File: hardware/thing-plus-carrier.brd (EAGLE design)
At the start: 160 x 100 mm, 8 parts, among them J1 THING_PLUS, U1 OKI-78SR-5/1.5-W36H-C, U2 MCP2004A-E/SNSOIC8_4P9X3P9MC_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, U3 MICROSD-BREAKOUT

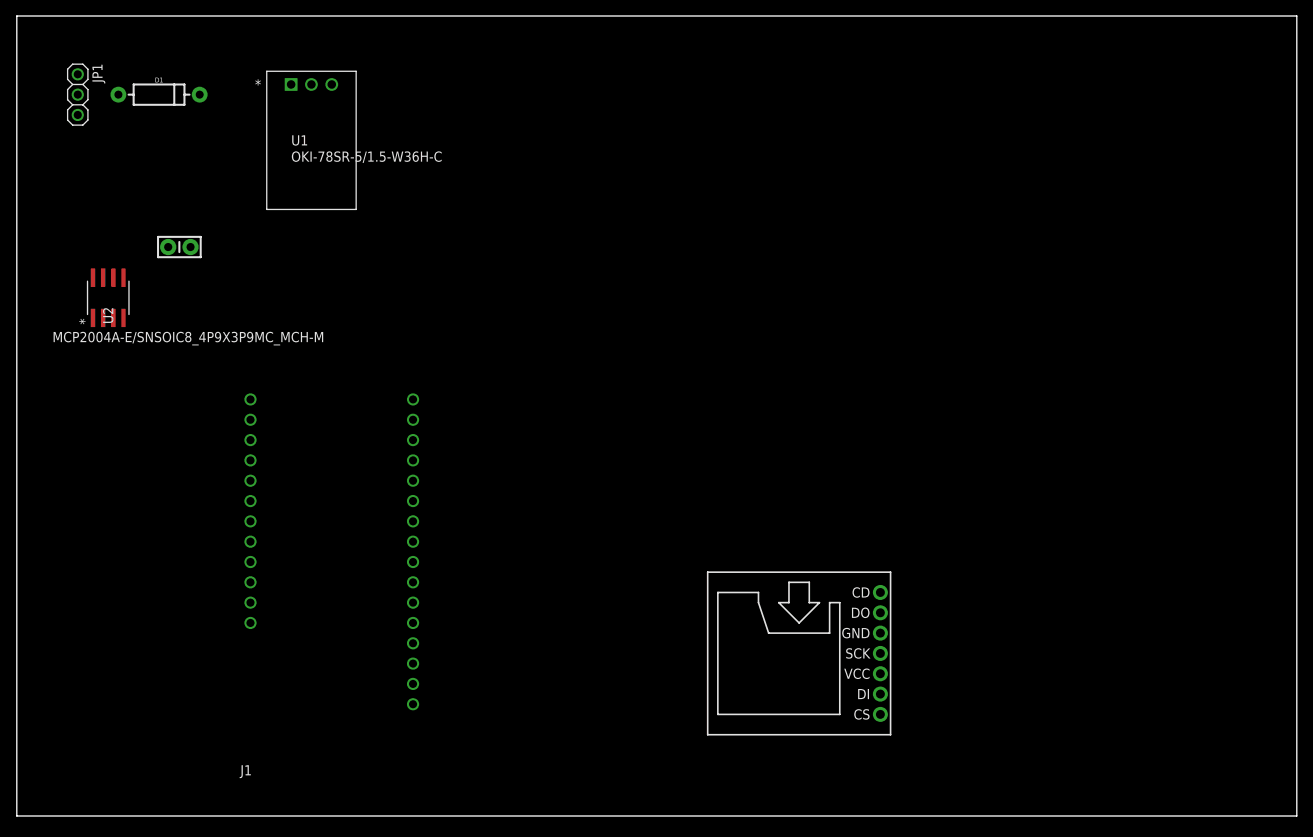
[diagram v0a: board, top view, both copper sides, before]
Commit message: Finished rev.1 board []~(￣▽￣)~* ; Updated docs
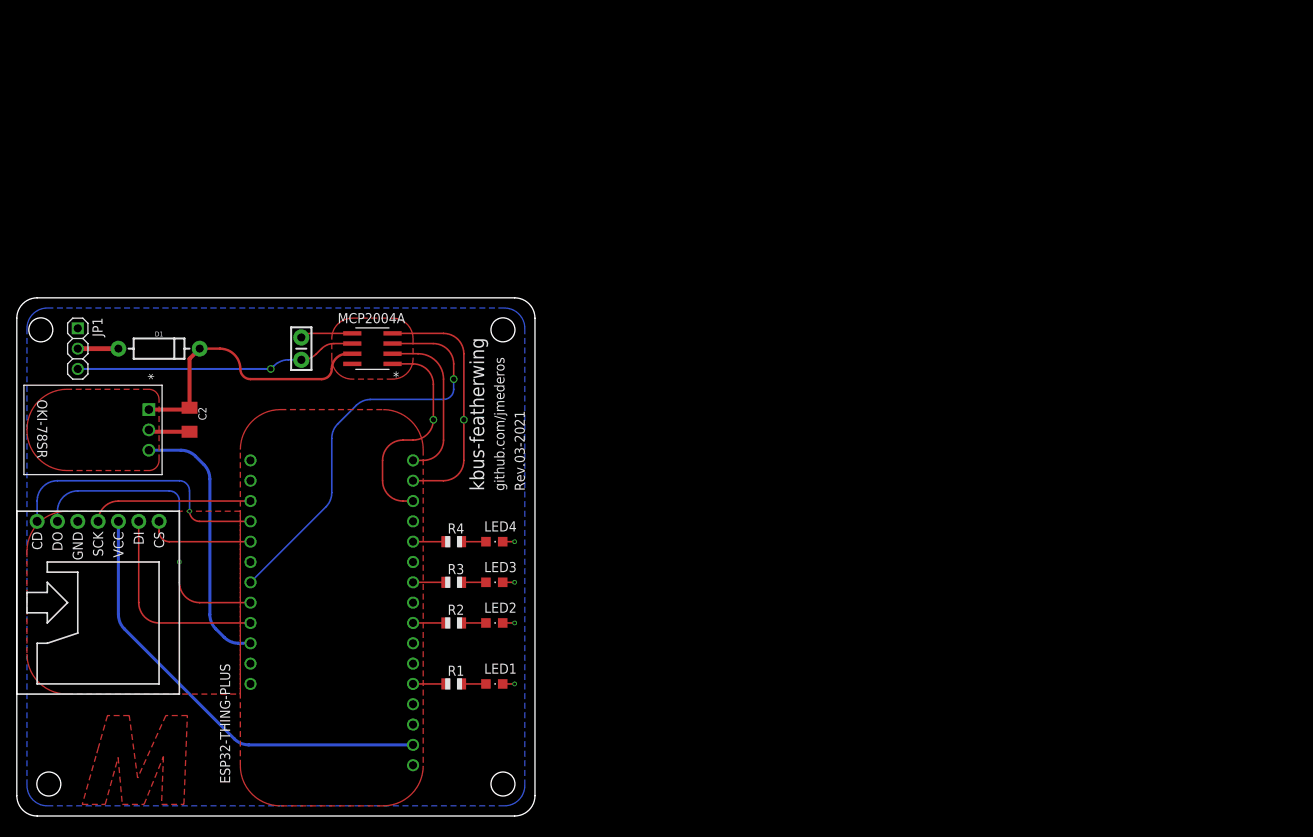
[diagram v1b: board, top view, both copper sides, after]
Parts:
- removed J1: THING_PLUS, SparkFun-Boards:THING_PLUS
- removed U1: OKI-78SR-5/1.5-W36H-C, kbus-feather-carrier-bom:OKI-78SR-5/1.5-W36H-C_MUR
- removed U2: MCP2004A-E/SNSOIC8_4P9X3P9MC_MCH-M, kbus-feather-carrier-bom:SOIC8_4P9X3P9MC_MCH-M
- added C2: 22uF, adafruit:C1206K
- added ESP32-THING-PLUS: THING_PLUS, SparkFun-Boards:THING_PLUS
- added LED1, LED2, LED3, LED4: (no value), adafruit:CHIPLED_0805
- added MCP2004A: MCP2004A-E/SNSOIC8_4P9X3P9MC_MCH-M, kbus-feather-carrier-bom:SOIC8_4P9X3P9MC_MCH-M
- added OKI-78SR: OKI-78SR-5/1.5-W36H-C, kbus-feather-carrier-bom:OKI-78SR-5/1.5-W36H-C_MUR
- added R1, R2, R3, R4: 1k, adafruit:R0805
- JP1: device adafruit:1X03 -> kbus-feather-carrier-bom:1X03
- U3: device SparkFun-Boards:MICROSD-BREAKOUT -> kbus-feather-carrier-bom:MICROSD-BREAKOUT
- moved U3 84.0 mm to (11.4, 24.1), turned to 90 degrees
- moved D1 31.8 mm to (17.8, 58.4)
- moved JP1 31.8 mm to (7.62, 58.4)
- moved C1 19.8 mm to (35.6, 58.4), turned to 90 degrees
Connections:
- new net N$1: ESP32-THING-PLUS.19, R3.1
- new net N$2: ESP32-THING-PLUS.24, R1.1
- new net N$3: ESP32-THING-PLUS.21, R2.1
- new net N$4: ESP32-THING-PLUS.17, R4.1
- new net N$5: LED4.A, R4.2
- new net N$6: LED3.A, R3.2
- new net N$7: LED2.A, R2.2
- new net N$8: LED1.A, R1.2
- net 12V: now also C2.1, MCP2004A.7, OKI-78SR.1; no longer U1.1, U2.7
- net 3V3: now also ESP32-THING-PLUS.27; no longer J1.27
- net 5V: now also ESP32-THING-PLUS.10, OKI-78SR.3; no longer J1.10, U1.3
- net CD: now also ESP32-THING-PLUS.4
- net CIPO: now also ESP32-THING-PLUS.8
- net COPI: now also ESP32-THING-PLUS.9
- net FAULT: now also ESP32-THING-PLUS.7, MCP2004A.3; no longer J1.7, U2.3
- net GND: now also C2.2, ESP32-THING-PLUS.25, ESP32-THING-PLUS.26, LED1.C, LED2.C, LED3.C, LED4.C, MCP2004A.5, OKI-78SR.2; no longer J1.25, J1.26, U1.2, U2.5
- net K-BUS: now also MCP2004A.6; no longer U2.6
- net RX: now also ESP32-THING-PLUS.15, MCP2004A.1; no longer J1.15, U2.1
- net SCK: now also ESP32-THING-PLUS.3
- net SD-CS: now also ESP32-THING-PLUS.5
- net TRX-CS: now also ESP32-THING-PLUS.13, MCP2004A.2; no longer J1.3, U2.2
- net TX: now also ESP32-THING-PLUS.14, MCP2004A.4; no longer J1.14, U2.4
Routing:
- net 3V3: track 0.00 -> 55.5 mm
- net FAULT: track 0.00 -> 52.0 mm, vias 0 -> 1
- net CIPO: track 0.00 -> 38.2 mm, vias 0 -> 1
- net 12V: track 0.00 -> 35.4 mm
- net K-BUS: track 0.00 -> 35.2 mm, vias 0 -> 1
- net CD: track 0.00 -> 33.9 mm, vias 0 -> 1
- net 5V: track 0.00 -> 33.2 mm
- net TX: track 0.00 -> 30.7 mm, vias 0 -> 1
- net RX: track 0.00 -> 26.5 mm, vias 0 -> 1
- net COPI: track 0.00 -> 25.2 mm
- net TRX-CS: track 0.00 -> 20.2 mm
- net SCK: track 0.00 -> 20.1 mm
- net GND: track 0.00 -> 17.6 mm, vias 0 -> 4
- net SD-CS: track 0.00 -> 13.2 mm
- net VBAT: track 0.00 -> 5.08 mm
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- added copper zone on layer 1, net GND
- added copper zone on layer 16, net GND
- added copper zone on layer 1, net N$9
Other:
- board size 160 x 100 mm -> 64.8 x 64.8 mm
- board text added: "Rev.03-2021"
- board text added: "github.com/jmederos"
- board text added: "kbus-featherwing"
